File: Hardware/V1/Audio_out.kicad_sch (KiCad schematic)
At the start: 30 parts, among them J0 0, J1 SJ2-3514A-SMT-TR, J2 0, Q1 BC817-25-QVL

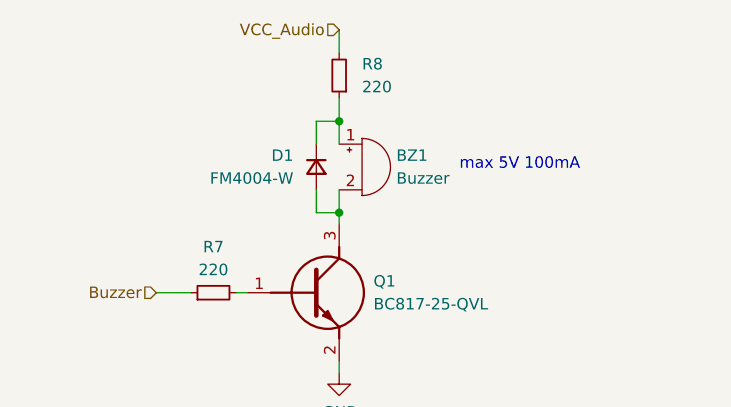
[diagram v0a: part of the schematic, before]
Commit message: motherboard update
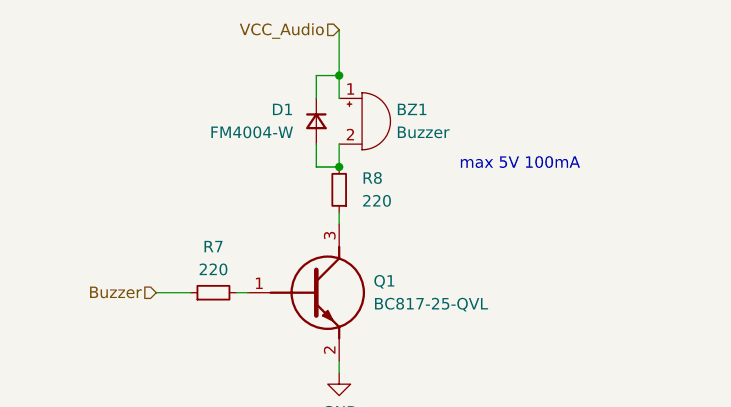
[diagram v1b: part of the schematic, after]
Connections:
- net VCC_Audio: now also BZ1.1 (+), D1.1 (K); no longer R8.2
- net at BZ1.2 (-), D1.2 (A): now also R8.2; no longer Q1.3 (C)
- new net: Q1.3 (C), R8.1
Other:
- moved on the sheet: BZ1, D1, R8
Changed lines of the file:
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@@
 	)
 	(junction
-		(at 48.26 29.21)
+		(at 48.26 24.13)
 		(diameter 0)
 		(color 0 0 0 0)
@@
 	)
 	(junction
-		(at 58.42 90.17)
+		(at 48.26 34.29)
 		(diameter 0)
 		(color 0 0 0 0)
 	)
 	(junction
-		(at 60.96 170.18)
+		(at 58.42 90.17)
 		(diameter 0)
 		(color 0 0 0 0)
 	)
 	(junction
-		(at 91.44 157.48)
+		(at 60.96 170.18)
 		(diameter 0)
 		(color 0 0 0 0)
 	)
 	(junction
-		(at 50.8 152.4)
+		(at 91.44 157.48)
 		(diameter 0)
 		(color 0 0 0 0)
 	)
 	(junction
-		(at 48.26 39.37)
+		(at 50.8 152.4)
 		(diameter 0)
 		(color 0 0 0 0)
@@
 	(wire
 		(pts
-			(xy 48.26 19.05) (xy 48.26 21.59)
+			(xy 48.26 19.05) (xy 48.26 24.13)
 		)
 		(stroke
@@
 	(wire
 		(pts
-			(xy 45.72 29.21) (xy 48.26 29.21)
+			(xy 45.72 24.13) (xy 48.26 24.13)
 		)
 		(stroke
@@
 	(wire
 		(pts
-			(xy 48.26 39.37) (xy 48.26 40.64)
-		)
-		(stroke
-			(width 0)
-			(type default)
-		)
-	)
-	(wire
-		(pts
 			(xy 49.53 90.17) (xy 58.42 90.17)
 		)
@@
 	(wire
 		(pts
-			(xy 45.72 36.83) (xy 45.72 39.37)
-		)
-		(stroke
-			(width 0)
-			(type default)
-		)
-	)
-	(wire
-		(pts
-			(xy 48.26 26.67) (xy 48.26 29.21)
+			(xy 45.72 31.75) (xy 45.72 34.29)
 		)
 		(stroke
@@
 	(wire
 		(pts
-			(xy 48.26 29.21) (xy 48.26 31.75)
+			(xy 48.26 24.13) (xy 48.26 26.67)
 		)
 		(stroke
@@
 	(wire
 		(pts
-			(xy 45.72 39.37) (xy 48.26 39.37)
+			(xy 45.72 34.29) (xy 48.26 34.29)
 		)
 		(stroke
@@
 	(wire
 		(pts
+			(xy 48.26 39.37) (xy 48.26 40.64)
+		)
+		(stroke
+			(width 0)
+			(type default)
+		)
+	)
+	(wire
+		(pts
 			(xy 58.42 113.03) (xy 62.23 113.03)
 		)
@@
 	(wire
 		(pts
-			(xy 45.72 31.75) (xy 45.72 29.21)
+			(xy 45.72 26.67) (xy 45.72 24.13)
 		)
 		(stroke
@@
 	(wire
 		(pts
-			(xy 48.26 36.83) (xy 48.26 39.37)
+			(xy 48.26 31.75) (xy 48.26 34.29)
 		)
 		(stroke
@@
 	(symbol
 		(lib_id "Device:Buzzer")
-		(at 50.8 34.29 0)
+		(at 50.8 29.21 0)
 		(unit 1)
 		(exclude_from_sim no)
@@
 		(fields_autoplaced yes)
 		(property "Reference" "BZ1"
-			(at 54.61 33.0199 0)
+			(at 54.61 27.9399 0)
 			(effects
 				(font
@@
 		)
 		(property "Value" "Buzzer"
-			(at 54.61 35.5599 0)
+			(at 54.61 30.4799 0)
 			(effects
 				(font
@@
 		)
 		(property "Footprint" "CMT052575SMTTR"
-			(at 50.165 31.75 90)
+			(at 50.165 26.67 90)
 			(effects
 				(font
@@
 		)
 		(property "Datasheet" "https://datasheet.datasheetarchive.com/originals/distributors/Datasheets_SAMA/202edec26f194914f30bb21e54dbec55.pdf"
-			(at 50.165 31.75 90)
+			(at 50.165 26.67 90)
 			(effects
 				(font
@@
 		)
 		(property "Description" "Buzzer, polarized"
-			(at 50.8 34.29 0)
+			(at 50.8 29.21 0)
 			(effects
 				(font
@@
 	(symbol
 		(lib_id "Device:D_Small")
-		(at 45.72 34.29 90)
+		(at 45.72 29.21 90)
 		(mirror x)
 		(unit 1)
@@
 		(dnp no)
 		(property "Reference" "D1"
-			(at 43.18 33.0199 90)
+			(at 43.18 27.9399 90)
 			(effects
 				(font
@@
 		)
 		(property "Value" "FM4004-W"
-			(at 43.18 35.5599 90)
+			(at 43.18 30.4799 90)
 			(effects
 				(font
@@
 		)
 		(property "Footprint" "DIONM5025X231N"
-			(at 45.72 34.29 90)
+			(at 45.72 29.21 90)
 			(effects
 				(font
@@
 		)
 		(property "Datasheet" "~"
-			(at 45.72 34.29 90)
+			(at 45.72 29.21 90)
 			(effects
 				(font
@@
 		)
 		(property "Description" "Diode, small symbol"
-			(at 45.72 34.29 0)
+			(at 45.72 29.21 0)
 			(effects
 				(font
@@
 		)
 		(property "Height" "2.31"
-			(at 443.18 45.72 0)
+			(at 443.18 40.64 0)
 			(effects
 				(font
@@
 		)
 		(property "Mouser Part Number" "583-FM4004"
-			(at 543.18 45.72 0)
+			(at 543.18 40.64 0)
 			(effects
 				(font
@@
 		)
 		(property "Mouser Price/Stock" "https://www.mouser.co.uk/ProductDetail/Rectron/FM4004-W?qs=Iw9Ubr57Px3IHNH1bE4l9w%3D%3D"
-			(at 643.18 45.72 0)
+			(at 643.18 40.64 0)
 			(effects
 				(font
@@
 		)
 		(property "Manufacturer_Name" "Rectron"
-			(at 743.18 45.72 0)
+			(at 743.18 40.64 0)
 			(effects
 				(font
@@
 		)
 		(property "Manufacturer_Part_Number" "FM4004-W"
-			(at 843.18 45.72 0)
+			(at 843.18 40.64 0)
 			(effects
 				(font
@@
 		)
 		(property "Sim.Device" "D"
-			(at 45.72 34.29 0)
+			(at 45.72 29.21 0)
 			(effects
 				(font
@@
 		)
 		(property "Sim.Pins" "1=K 2=A"
-			(at 45.72 34.29 0)
+			(at 45.72 29.21 0)
 			(effects
 				(font
@@
 	(symbol
 		(lib_id "Device:R_Small")
-		(at 48.26 24.13 180)
+		(at 48.26 36.83 180)
 		(unit 1)
 		(exclude_from_sim no)
@@
 		(fields_autoplaced yes)
 		(property "Reference" "R8"
-			(at 50.8 22.8599 0)
+			(at 50.8 35.5599 0)
 			(effects
 				(font
@@
 		)
 		(property "Value" "220"
-			(at 50.8 25.3999 0)
+			(at 50.8 38.0999 0)
 			(effects
 				(font
@@
 		)
 		(property "Footprint" "Resistor_SMD:R_0603_1608Metric"
-			(at 48.26 24.13 0)
+			(at 48.26 36.83 0)
 			(effects
 				(font
@@
 		)
 		(property "Datasheet" "~"
-			(at 48.26 24.13 0)
+			(at 48.26 36.83 0)
 			(effects
 				(font
@@
 		)
 		(property "Description" "Resistor, small symbol"
-			(at 48.26 24.13 0)
+			(at 48.26 36.83 0)
 			(effects
 				(font
